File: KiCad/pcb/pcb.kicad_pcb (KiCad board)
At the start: 2 copper layers, 65 x 98.4 mm, 19 parts, among them J1 Screw_Terminal_01x06, J2 Screw_Terminal_01x03, J3 Screw_Terminal_01x06, U1 OKY3504-1, U2 Tauno_Oled_096_SSD1306, U3 PC817

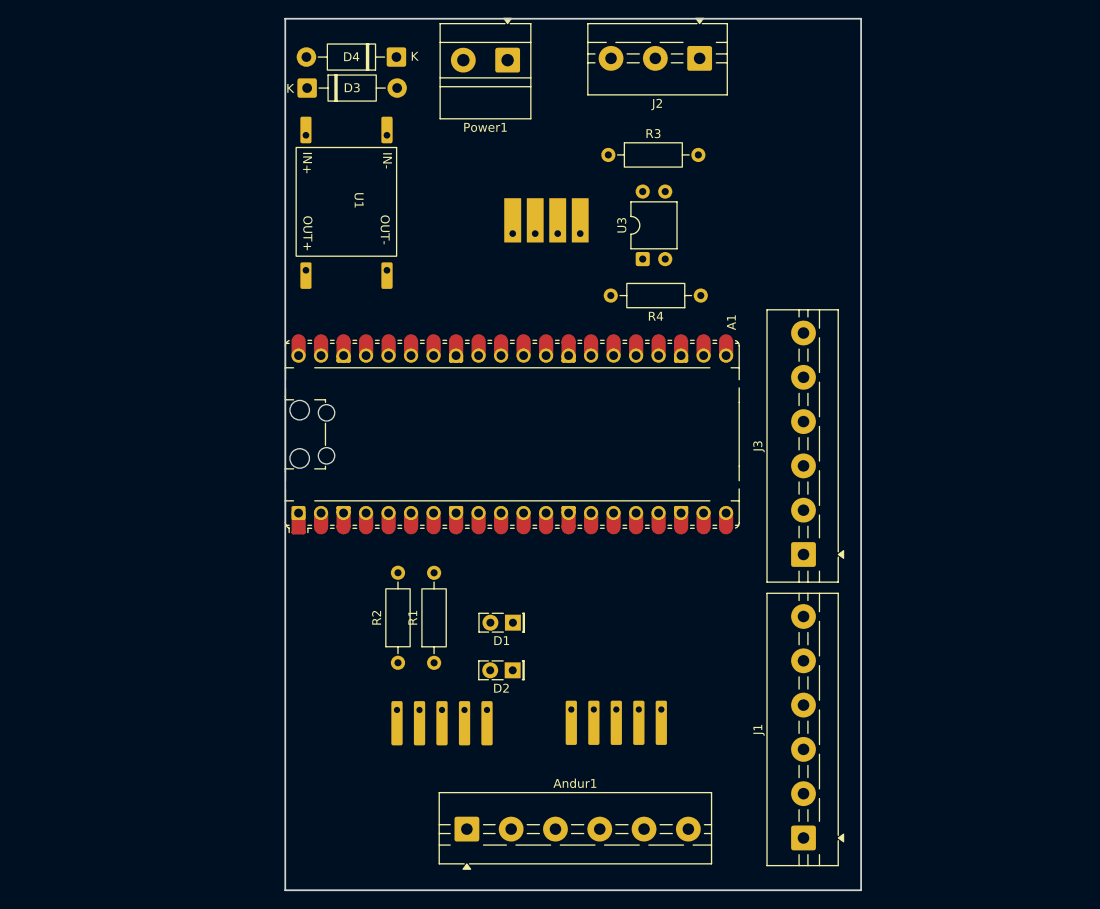
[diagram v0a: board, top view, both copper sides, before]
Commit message: kicad files
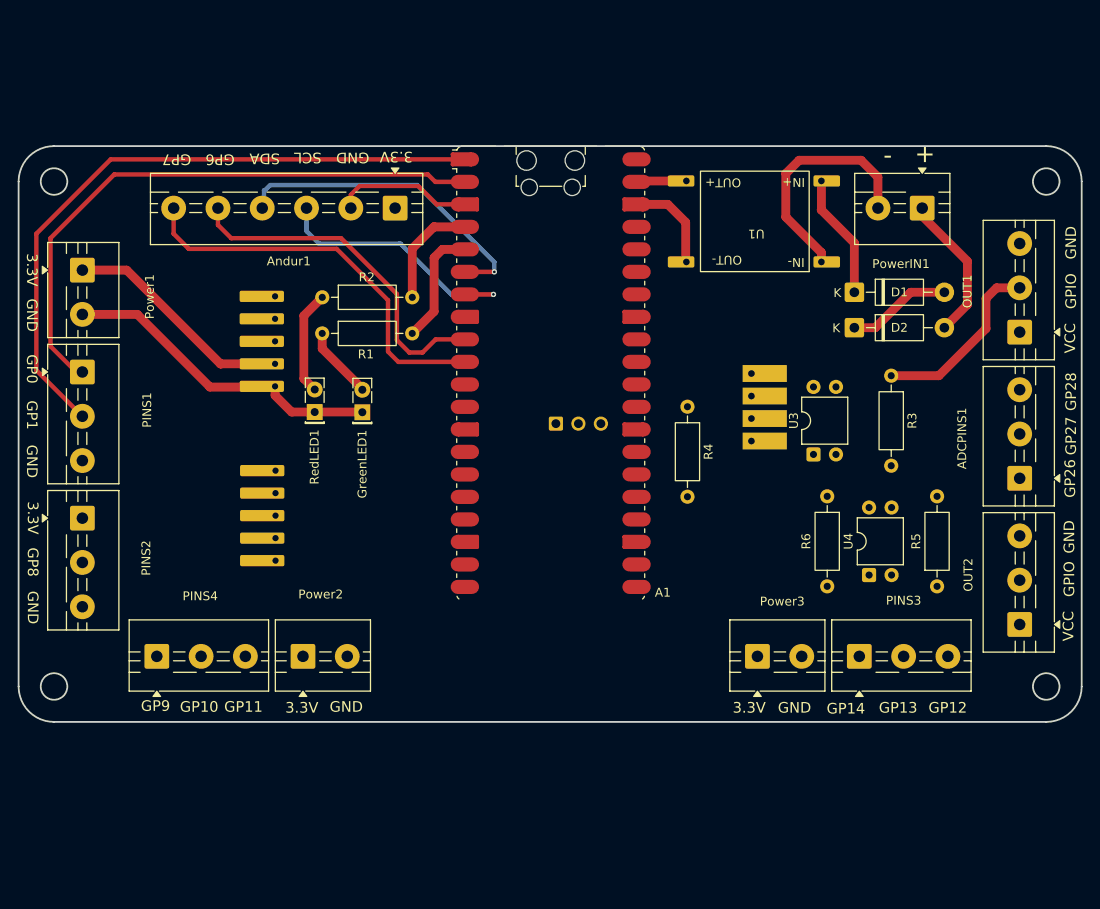
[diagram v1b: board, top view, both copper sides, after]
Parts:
- removed J1, J3: Screw_Terminal_01x06, TerminalBlock:TerminalBlock_MaiXu_MX126-5.0-06P_1x06_P5.00mm
- added ADCPINS1: Screw_Terminal_01x03, TerminalBlock:TerminalBlock_MaiXu_MX126-5.0-03P_1x03_P5.00mm, F.Cu at (155.4, 131.4)
- added OUT2: Screw_Terminal_01x03, TerminalBlock:TerminalBlock_MaiXu_MX126-5.0-03P_1x03_P5.00mm, F.Cu at (155.4, 147.9)
- added PINS1: Screw_Terminal_01x03, TerminalBlock:TerminalBlock_MaiXu_MX126-5.0-03P_1x03_P5.00mm, F.Cu at (49.6, 119.4)
- added PINS2: Screw_Terminal_01x03, TerminalBlock:TerminalBlock_MaiXu_MX126-5.0-03P_1x03_P5.00mm, F.Cu at (49.6, 135.9)
- added PINS3: Screw_Terminal_01x03, TerminalBlock:TerminalBlock_MaiXu_MX126-5.0-03P_1x03_P5.00mm, F.Cu at (137.3, 151.5)
- added PINS4: Screw_Terminal_01x03, TerminalBlock:TerminalBlock_MaiXu_MX126-5.0-03P_1x03_P5.00mm, F.Cu at (58.0, 151.5)
- added Power1: Screw_Terminal_01x02, TerminalBlock:TerminalBlock_MaiXu_MX126-5.0-02P_1x02_P5.00mm, F.Cu at (49.6, 107.9)
- added Power2: Screw_Terminal_01x02, TerminalBlock:TerminalBlock_MaiXu_MX126-5.0-02P_1x02_P5.00mm, F.Cu at (74.5, 151.5)
- added Power3: Screw_Terminal_01x02, TerminalBlock:TerminalBlock_MaiXu_MX126-5.0-02P_1x02_P5.00mm, F.Cu at (125.8, 151.5)
- added R5: 10K, Resistor_THT:R_Axial_DIN0207_L6.3mm_D2.5mm_P10.16mm_Horizontal, F.Cu at (146.1, 143.6)
- added R6: 470, Resistor_THT:R_Axial_DIN0207_L6.3mm_D2.5mm_P10.16mm_Horizontal, F.Cu at (133.7, 133.4)
- added U4: PC817, Package_DIP:DIP-4_W7.62mm, F.Cu at (138.4, 142.3)
- A1: footprint Module:RaspberryPi_Pico_Common_Unspecified -> Module:RaspberryPi_Pico_W_SMD_HandSolder
- PowerIN1: renamed from Power1; footprint TerminalBlock_MetzConnect:TerminalBlock_MetzConnect_Type011_RT05502HBLC_1x02_P5.00mm_Horizontal -> TerminalBlock:TerminalBlock_MaiXu_MX126-5.0-02P_1x02_P5.00mm
- moved Andur1 70.6 mm to (84.9, 100.9), turned to 180 degrees
- moved D1 65.9 mm to (136.7, 110.4)
- moved Right1 60.4 mm to (66.3, 103.2), turned to 180 degrees
- moved D2 60.0 mm to (136.7, 114.4), turned to 0 degrees
- moved U1 51.1 mm to (133.0, 107.0), turned to 180 degrees
- moved Left1 50.2 mm to (66.3, 122.9), turned to 180 degrees
- moved PowerIN1 49.7 mm to (144.4, 100.9)
- moved OUT1 47.5 mm to (155.4, 114.9), turned to 90 degrees
- moved R2 42.1 mm to (76.7, 111.0), turned to 0 degrees
- moved R3 40.5 mm to (140.9, 119.8), turned to -90 degrees
- moved R1 39.3 mm to (76.7, 115.0), turned to 0 degrees
- moved U2 37.5 mm to (130.2, 123.4), turned to 90 degrees
- moved RedLED1 36.7 mm to (75.8, 123.9), turned to 90 degrees
- moved U3 29.3 mm to (132.1, 128.7)
- moved GreenLED1 29.2 mm to (81.2, 123.9), turned to 90 degrees
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- renumbered D3 to D1, D4 to D2, D1 to GreenLED1, J2 to OUT1, D2 to RedLED1
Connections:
- A1 pad 1: /UART TX -> GPIO0
- A1 pad 2: /UART RX -> GPIO1
- A1 pad 31: unconnected-(A1-GPIO26_ADC0-Pad31) -> Net-(A1-GPIO26_ADC0)
- A1 pad 32: unconnected-(A1-GPIO27_ADC1-Pad32) -> Net-(A1-GPIO27_ADC1)
- A1 pad 34: unconnected-(A1-GPIO28_ADC2-Pad34) -> Net-(A1-GPIO28_ADC2)
- U2 pad 3: /SCL -> unconnected-(U2-SCL-Pad3)
- U2 pad 4: /SDA -> unconnected-(U2-SDA-Pad4)
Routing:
- net GPIO0: track 0.00 -> 74.6 mm
- net GPIO1: track 0.00 -> 68.2 mm
- net GND: track 0.00 -> 63.4 mm
- net Net-(A1-GPIO7): track 0.00 -> 45.2 mm
- net Net-(A1-GPIO6): track 0.00 -> 39.4 mm
- net /SDA: track 0.00 -> 36.4 mm, vias 0 -> 1
- net /SCL: track 0.00 -> 29.9 mm, vias 0 -> 1
- net Net-(PowerIN1-Pin_2): track 0.00 -> 27.0 mm
- net +3.3V: track 0.00 -> 26.1 mm
- net /External_GPIO: track 0.00 -> 20.6 mm
- net Net-(D2-A): track 0.00 -> 16.7 mm
- net Net-(D1-K): track 0.00 -> 14.1 mm
- net /Green_LED: track 0.00 -> 13.4 mm
- net /Red_LED: track 0.00 -> 12.5 mm
- net Net-(D1-A): track 0.00 -> 11.8 mm
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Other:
- board size 65 x 98.4 mm -> 120 x 65 mm
- board text added: "+"
- board text added: "-"
- board text added: "3.3V"
- board text added: "GND"
- board text added: "GP0"
- board text added: "GP1"
- board text added: "GP10"
- board text added: "GP11"
- board text added: "GP12"
- board text added: "GP13"
- board text added: "GP14"
- board text added: "GP26"
- board text added: "GP27"
- board text added: "GP28"
- board text added: "GP6"
- board text added: "GP7"
- board text added: "GP8"
- board text added: "GP9"
- board text added: "GPIO"
- board text added: "SCL"
- board text added: "SDA"
- board text added: "VCC"
